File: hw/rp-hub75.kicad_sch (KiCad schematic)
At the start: 39 parts, among them J1 Display Connector, J2 USB_C_Receptacle_USB2.0_16P, J3 Screw_Terminal_01x02, J5 USB_A, J6 Conn_01x10, J7 Conn_01x05, J8 Conn_01x04, SW1 SW_Push, U1 AMS1117-3.3, U2 RP2350_60QFN, U3 ZD25WQ80CTIGT, Y1 TXM12M0004322CBCDO00T

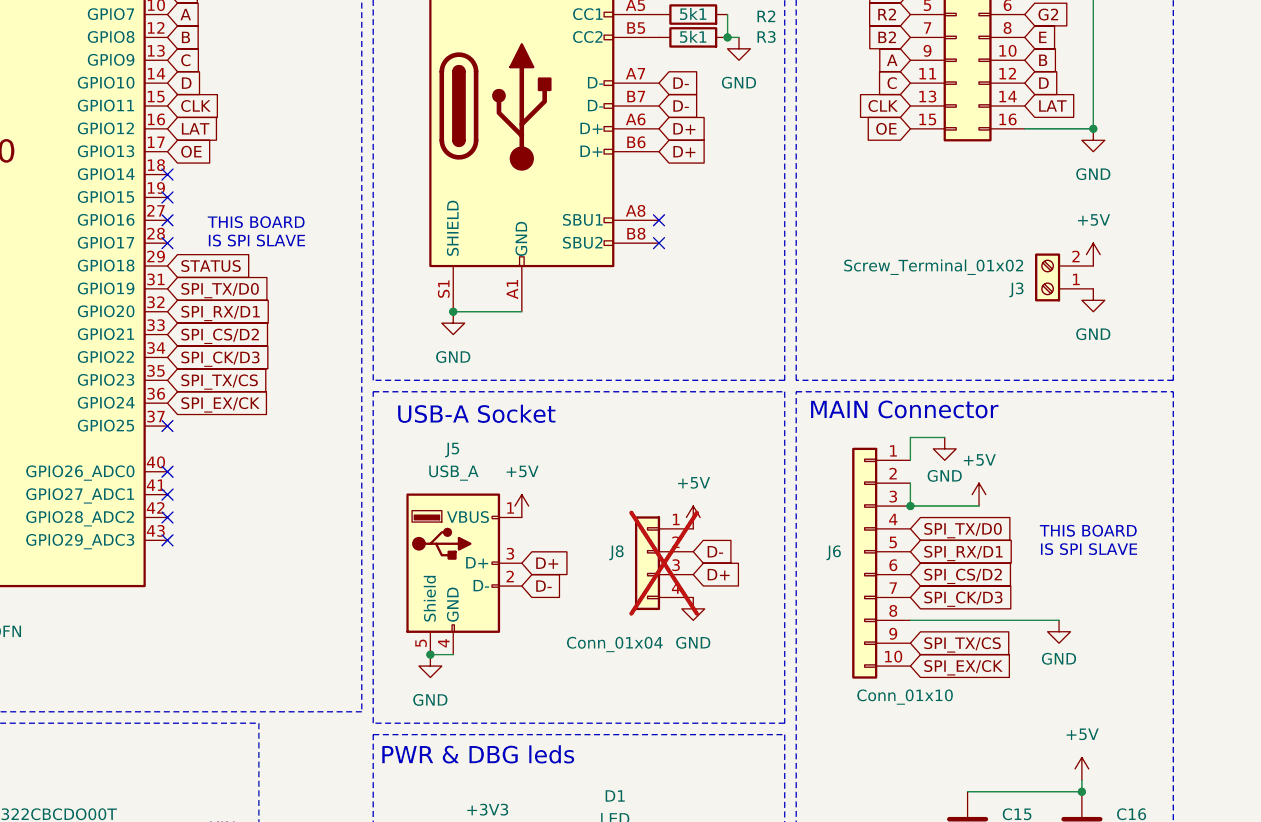
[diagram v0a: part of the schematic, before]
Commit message: v1.6
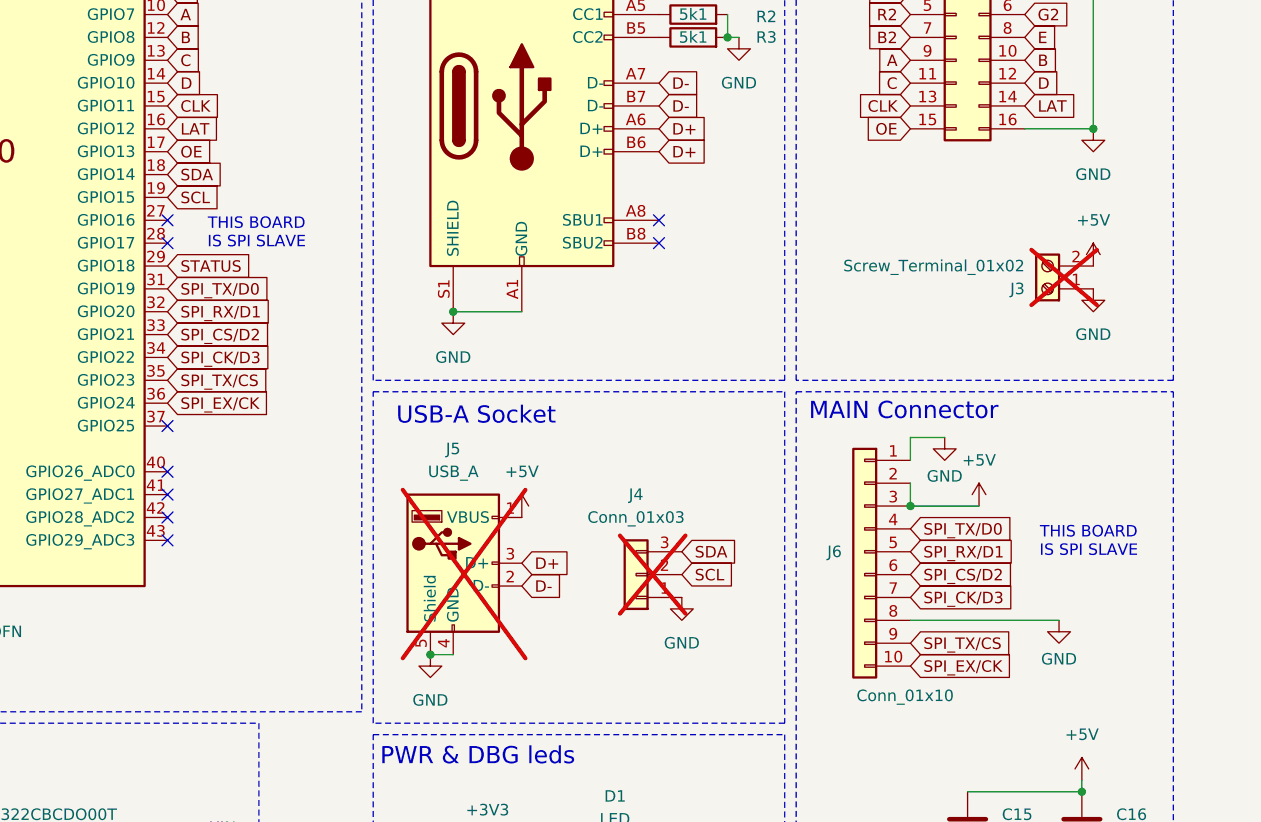
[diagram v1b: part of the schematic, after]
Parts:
- removed J8: Conn_01x04, Connector_PinHeader_2.54mm:PinHeader_1x04_P2.54mm_Vertical, symbol Connector_Generic:Conn_01x04
- added J4: Conn_01x03, Connector_PinHeader_2.54mm:PinHeader_1x03_P2.54mm_Vertical, symbol Connector_Generic:Conn_01x03
- J3, J5: now not fitted
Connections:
- net GND: now also J4.1 (Pin_1)
- net SDA: now reaches U2.18 (GPIO14)
- net SDA: now also J4.3 (Pin_3)
- net SCL: now reaches U2.19 (GPIO15)
- net SCL: now also J4.2 (Pin_2)
- no-connect marks 11 -> 9
